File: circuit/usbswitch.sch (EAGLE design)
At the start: 11 parts, among them IC1 TINY25, Q2 BSA223SP

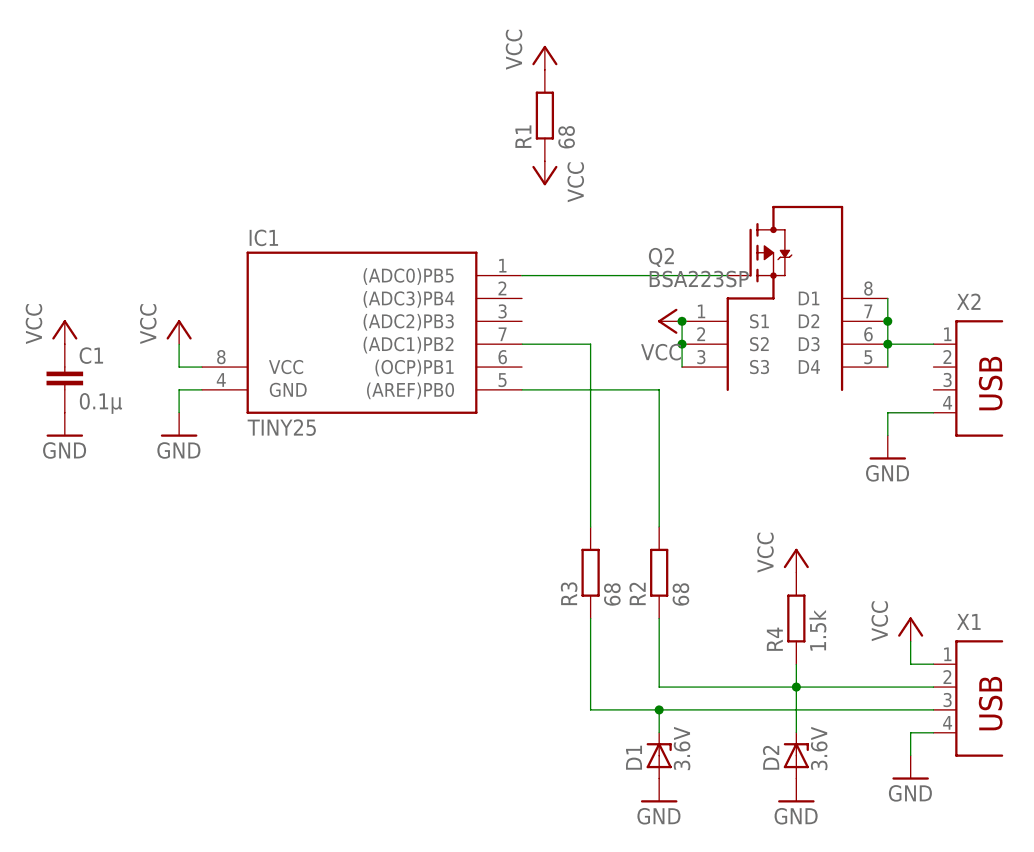
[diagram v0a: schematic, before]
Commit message: cleanup
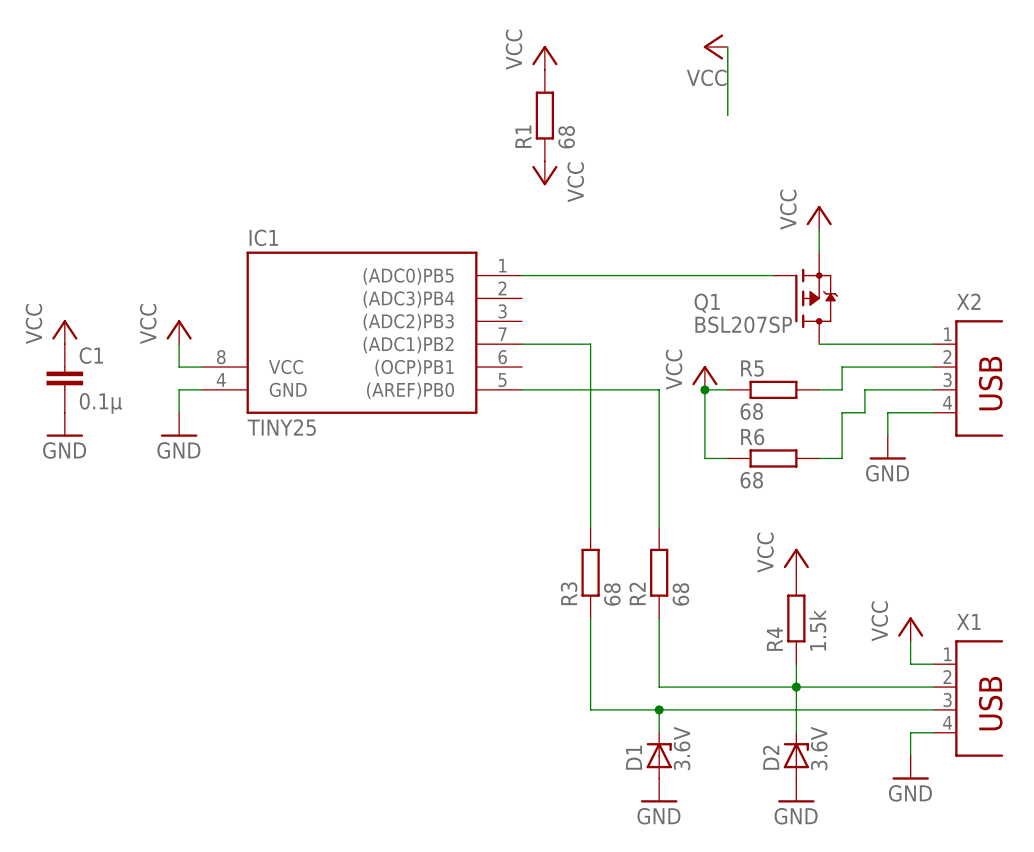
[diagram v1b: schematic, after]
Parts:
- removed Q2: BSA223SP, irf:BSA223SP
- added Q1: BSL207SP, irf:BSL207SP
- added R5, R6: 68, resistor:R-EU_R1206
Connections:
- new net N$3: R5.2, X2.2
- new net N$8: R6.2, X2.3
- net N$1: now also Q1.G; no longer Q2.G
- net N$2: now also Q1.D; no longer Q2.D1, Q2.D2, Q2.D3, Q2.D4
- net VCC: now also Q1.S, R5.1, R6.1; no longer Q2.S1, Q2.S2, Q2.S3
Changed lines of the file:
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@@
 <part name="GND7" library="supply1" deviceset="GND" device=""/>
 <part name="C1" library="resistor" deviceset="C-EU" device="C1206" value="0.1µ"/>
-<part name="Q2" library="irf" deviceset="BSA223SP" device=""/>
 <part name="R1" library="resistor" deviceset="R-EU_" device="R1206" value="68"/>
 <part name="P+5" library="supply1" deviceset="VCC" device=""/>
 <part name="P+7" library="supply1" deviceset="VCC" device=""/>
+<part name="Q1" library="irf" deviceset="BSL207SP" device=""/>
+<part name="P+8" library="supply1" deviceset="VCC" device=""/>
+<part name="R5" library="resistor" deviceset="R-EU_" device="R1206" value="68"/>
+<part name="R6" library="resistor" deviceset="R-EU_" device="R1206" value="68"/>
+<part name="P+9" library="supply1" deviceset="VCC" device=""/>
 </parts>
 <sheets>
@@
 <instance part="P+1" gate="VCC" x="38.1" y="71.12"/>
 <instance part="P+2" gate="VCC" x="119.38" y="38.1"/>
-<instance part="P+3" gate="VCC" x="91.44" y="71.12" rot="R90"/>
+<instance part="P+3" gate="VCC" x="96.52" y="101.6" rot="R90"/>
 <instance part="GND1" gate="1" x="38.1" y="58.42"/>
 <instance part="GND2" gate="1" x="119.38" y="20.32"/>
@@
 <instance part="GND7" gate="1" x="25.4" y="58.42"/>
 <instance part="C1" gate="G$1" x="25.4" y="66.04"/>
-<instance part="Q2" gate="G$1" x="101.6" y="78.74"/>
 <instance part="R1" gate="G$1" x="78.74" y="93.98" rot="R90"/>
 <instance part="P+5" gate="VCC" x="78.74" y="101.6"/>
 <instance part="P+7" gate="VCC" x="78.74" y="86.36" rot="R180"/>
+<instance part="Q1" gate="G$1" x="106.68" y="73.66"/>
+<instance part="P+8" gate="VCC" x="109.22" y="83.82"/>
+<instance part="R5" gate="G$1" x="104.14" y="63.5"/>
+<instance part="R6" gate="G$1" x="104.14" y="55.88"/>
+<instance part="P+9" gate="VCC" x="96.52" y="66.04"/>
 </instances>
 <busses>
@@
 </segment>
 <segment>
-<pinref part="Q2" gate="G$1" pin="S1"/>
 <pinref part="P+3" gate="VCC" pin="VCC"/>
-<pinref part="Q2" gate="G$1" pin="S3"/>
-<wire x1="93.98" y1="71.12" x2="93.98" y2="68.58" width="0.1524" layer="91"/>
-<junction x="93.98" y="71.12"/>
-<pinref part="Q2" gate="G$1" pin="S2"/>
-<wire x1="93.98" y1="68.58" x2="93.98" y2="66.04" width="0.1524" layer="91"/>
-<junction x="93.98" y="68.58"/>
+<wire x1="99.06" y1="101.6" x2="99.06" y2="93.98" width="0.1524" layer="91"/>
 </segment>
 <segment>
@@
 <pinref part="P+7" gate="VCC" pin="VCC"/>
 </segment>
+<segment>
+<pinref part="Q1" gate="G$1" pin="S"/>
+<pinref part="P+8" gate="VCC" pin="VCC"/>
+<wire x1="109.22" y1="81.28" x2="109.22" y2="78.74" width="0.1524" layer="91"/>
+</segment>
+<segment>
+<pinref part="R6" gate="G$1" pin="1"/>
+<wire x1="99.06" y1="55.88" x2="96.52" y2="55.88" width="0.1524" layer="91"/>
+<wire x1="96.52" y1="55.88" x2="96.52" y2="63.5" width="0.1524" layer="91"/>
+<pinref part="R5" gate="G$1" pin="1"/>
+<wire x1="96.52" y1="63.5" x2="99.06" y2="63.5" width="0.1524" layer="91"/>
+<pinref part="P+9" gate="VCC" pin="VCC"/>
+<junction x="96.52" y="63.5"/>
+</segment>
 </net>
 <net name="N$1" class="0">
 <segment>
 <pinref part="IC1" gate="G$1" pin="(ADC0)PB5"/>
-<wire x1="99.06" y1="76.2" x2="76.2" y2="76.2" width="0.1524" layer="91"/>
-<pinref part="Q2" gate="G$1" pin="G"/>
+<wire x1="104.14" y1="76.2" x2="76.2" y2="76.2" width="0.1524" layer="91"/>
+<pinref part="Q1" gate="G$1" pin="G"/>
 </segment>
 </net>
@@
 <net name="N$2" class="0">
 <segment>
-<pinref part="Q2" gate="G$1" pin="D1"/>
-<pinref part="Q2" gate="G$1" pin="D4"/>
-<wire x1="116.84" y1="73.66" x2="116.84" y2="71.12" width="0.1524" layer="91"/>
-<pinref part="Q2" gate="G$1" pin="D2"/>
-<wire x1="116.84" y1="71.12" x2="116.84" y2="68.58" width="0.1524" layer="91"/>
-<junction x="116.84" y="71.12"/>
-<pinref part="Q2" gate="G$1" pin="D3"/>
-<wire x1="116.84" y1="68.58" x2="116.84" y2="66.04" width="0.1524" layer="91"/>
-<junction x="116.84" y="68.58"/>
+<pinref part="Q1" gate="G$1" pin="D"/>
 <pinref part="X2" gate="G$1" pin="1"/>
-<wire x1="116.84" y1="68.58" x2="121.92" y2="68.58" width="0.1524" layer="91"/>
-</segment>
-</net>
+<wire x1="109.22" y1="68.58" x2="121.92" y2="68.58" width="0.1524" layer="91"/>
+</segment>
+</net>
+<net name="N$3" class="0">
+<segment>
+<pinref part="R5" gate="G$1" pin="2"/>
+<wire x1="109.22" y1="63.5" x2="111.76" y2="63.5" width="0.1524" layer="91"/>
+<wire x1="111.76" y1="63.5" x2="111.76" y2="66.04" width="0.1524" layer="91"/>
+<pinref part="X2" gate="G$1" pin="2"/>
+<wire x1="111.76" y1="66.04" x2="121.92" y2="66.04" width="0.1524" layer="91"/>
+</segment>
+</net>
+<net name="N$8" class="0">
+<segment>
+<pinref part="R6" gate="G$1" pin="2"/>
+<wire x1="109.22" y1="55.88" x2="111.76" y2="55.88" width="0.1524" layer="91"/>
+<wire x1="111.76" y1="55.88" x2="111.76" y2="60.96" width="0.1524" layer="91"/>
+<wire x1="111.76" y1="60.96" x2="114.3" y2="60.96" width="0.1524" layer="91"/>
+<wire x1="114.3" y1="60.96" x2="114.3" y2="63.5" width="0.1524" layer="91"/>
+<pinref part="X2" gate="G$1" pin="3"/>
+<wire x1="114.3" y1="63.5" x2="121.92" y2="63.5" width="0.1524" layer="91"/>
+</segment>
+</net>
